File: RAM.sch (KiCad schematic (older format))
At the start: 9 parts

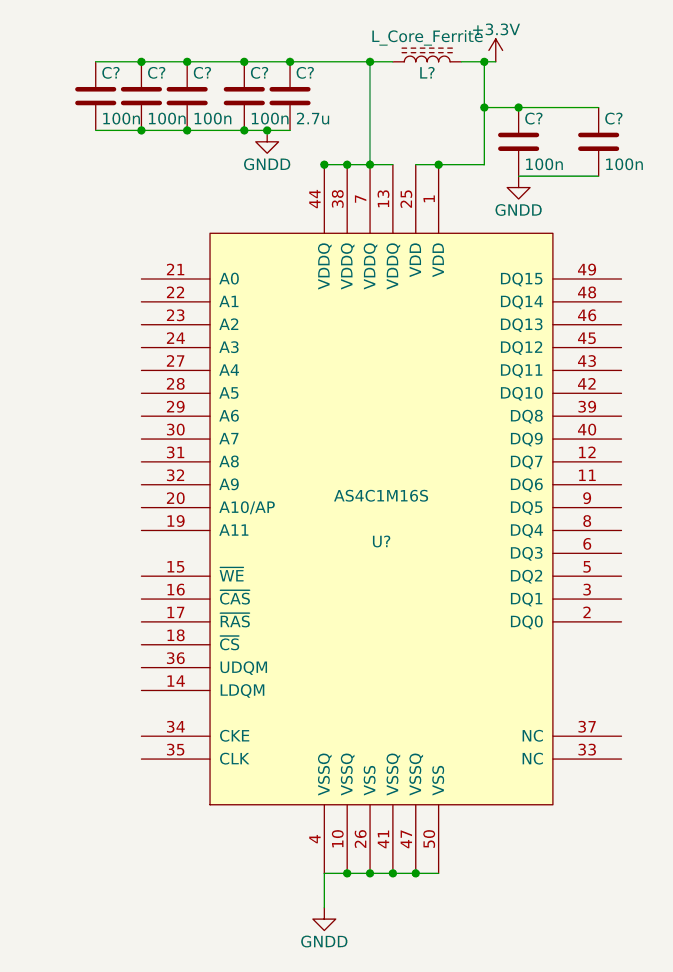
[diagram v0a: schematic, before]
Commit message: Minor fixes and the gitignore was removed
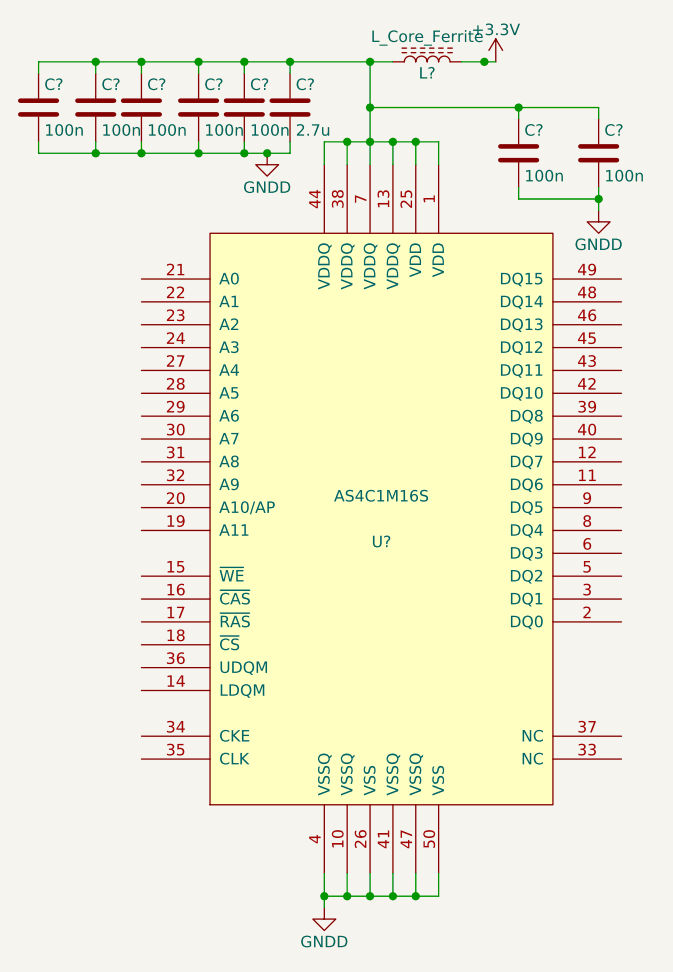
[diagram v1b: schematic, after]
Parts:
- added C?: 100n, symbol C
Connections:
- net +3V3: no longer C?.1, C?.1, U?.1 (VDD), U?.25 (VDD)
- net GNDD: now also C?.2
- net at C?.1, C?.1, C?.1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: now also C?.1, C?.1, U?.1 (VDD), U?.25 (VDD), C?.1
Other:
- moved on the sheet: C?
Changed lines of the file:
@@
 L C C?
 U 1 1 58E1D705
-P 4600 1350
-F 0 "C?" H 4625 1450 50  0000 L CNN
-F 1 "2.7u" H 4625 1250 50  0000 L CNN
-F 2 "" H 4638 1200 50  0001 C CNN
-F 3 "" H 4600 1350 50  0001 C CNN
-	1    4600 1350
+P 4600 1400
+F 0 "C?" H 4625 1500 50  0000 L CNN
+F 1 "2.7u" H 4625 1300 50  0000 L CNN
+F 2 "" H 4638 1250 50  0001 C CNN
+F 3 "" H 4600 1400 50  0001 C CNN
+	1    4600 1400
 	1    0    0    -1
 $EndComp
@@
 L C C?
 U 1 1 58E1D776
-P 4400 1350
-F 0 "C?" H 4425 1450 50  0000 L CNN
-F 1 "100n" H 4425 1250 50  0000 L CNN
-F 2 "" H 4438 1200 50  0001 C CNN
-F 3 "" H 4400 1350 50  0001 C CNN
-	1    4400 1350
+P 4400 1400
+F 0 "C?" H 4425 1500 50  0000 L CNN
+F 1 "100n" H 4425 1300 50  0000 L CNN
+F 2 "" H 4438 1250 50  0001 C CNN
+F 3 "" H 4400 1400 50  0001 C CNN
+	1    4400 1400
 	1    0    0    -1
 $EndComp
@@
 L GNDD #PWR?
 U 1 1 58E1D898
-P 4500 1500
-F 0 "#PWR?" H 4500 1250 50  0001 C CNN
-F 1 "GNDD" H 4500 1350 50  0000 C CNN
-F 2 "" H 4500 1500 50  0001 C CNN
-F 3 "" H 4500 1500 50  0001 C CNN
-	1    4500 1500
+P 4500 1600
+F 0 "#PWR?" H 4500 1350 50  0001 C CNN
+F 1 "GNDD" H 4500 1450 50  0000 C CNN
+F 2 "" H 4500 1600 50  0001 C CNN
+F 3 "" H 4500 1600 50  0001 C CNN
+	1    4500 1600
 	1    0    0    -1
 $EndComp
@@
 	4750 4900 4750 4750
 Wire Wire Line
-	4750 4750 5250 4750
-Connection ~ 4850 4750
-Connection ~ 4950 4750
-Connection ~ 5050 4750
-Connection ~ 5150 4750
-Wire Wire Line
 	5350 1200 5500 1200
 Wire Wire Line
-	3750 1200 5050 1200
+	3500 1200 5050 1200
 Connection ~ 4600 1200
-Wire Wire Line
-	4750 1650 5050 1650
 Wire Wire Line
 	4950 1650 4950 1200
 Connection ~ 4950 1200
-Wire Wire Line
-	5450 1650 5450 1200
 Connection ~ 5450 1200
-Wire Wire Line
-	3750 1500 4600 1500
-Connection ~ 4500 1500
-Connection ~ 4850 1650
+$Comp
+L C C?
+U 1 1 58E1DAA0
+P 3750 1400
+F 0 "C?" H 3775 1500 50  0000 L CNN
+F 1 "100n" H 3775 1300 50  0000 L CNN
+F 2 "" H 3788 1250 50  0001 C CNN
+F 3 "" H 3750 1400 50  0001 C CNN
+	1    3750 1400
+	1    0    0    -1
+$EndComp
+$Comp
+L C C?
+U 1 1 58E1DADF
+P 3950 1400
+F 0 "C?" H 3975 1500 50  0000 L CNN
+F 1 "100n" H 3975 1300 50  0000 L CNN
+F 2 "" H 3988 1250 50  0001 C CNN
+F 3 "" H 3950 1400 50  0001 C CNN
+	1    3950 1400
+	1    0    0    -1
+$EndComp
+$Comp
+L C C?
+U 1 1 58E1DB0D
+P 4200 1400
+F 0 "C?" H 4225 1500 50  0000 L CNN
+F 1 "100n" H 4225 1300 50  0000 L CNN
+F 2 "" H 4238 1250 50  0001 C CNN
+F 3 "" H 4200 1400 50  0001 C CNN
+	1    4200 1400
+	1    0    0    -1
+$EndComp
+Connection ~ 3950 1200
+Connection ~ 4400 1200
+$Comp
+L C C?
+U 1 1 58E1DD36
+P 5600 1600
+F 0 "C?" H 5625 1700 50  0000 L CNN
+F 1 "100n" H 5625 1500 50  0000 L CNN
+F 2 "" H 5638 1450 50  0001 C CNN
+F 3 "" H 5600 1600 50  0001 C CNN
+	1    5600 1600
+	1    0    0    -1
+$EndComp
+$Comp
+L GNDD #PWR?
+U 1 1 58E1DD7E
+P 5950 1850
+F 0 "#PWR?" H 5950 1600 50  0001 C CNN
+F 1 "GNDD" H 5950 1700 50  0000 C CNN
+F 2 "" H 5950 1850 50  0001 C CNN
+F 3 "" H 5950 1850 50  0001 C CNN
+	1    5950 1850
+	1    0    0    -1
+$EndComp
+$Comp
+L C C?
+U 1 1 58E1DDA1
+P 5950 1600
+F 0 "C?" H 5975 1700 50  0000 L CNN
+F 1 "100n" H 5975 1500 50  0000 L CNN
+F 2 "" H 5988 1450 50  0001 C CNN
+F 3 "" H 5950 1600 50  0001 C CNN
+	1    5950 1600
+	1    0    0    -1
+$EndComp
+Wire Wire Line
+	4950 1400 5950 1400
+Connection ~ 5600 1400
+Wire Wire Line
+	3750 1250 3750 1200
+Wire Wire Line
+	3950 1250 3950 1200
+Wire Wire Line
+	4400 1250 4400 1200
+Wire Wire Line
+	4600 1250 4600 1200
+Wire Wire Line
+	4600 1600 4600 1550
+Wire Wire Line
+	3500 1600 4600 1600
+Wire Wire Line
+	3750 1600 3750 1550
+Connection ~ 4500 1600
+Wire Wire Line
+	3950 1550 3950 1600
+Connection ~ 3950 1600
+Wire Wire Line
+	4400 1550 4400 1600
+Connection ~ 4400 1600
+Wire Wire Line
+	4200 1250 4200 1200
+Connection ~ 4200 1200
+Wire Wire Line
+	4200 1550 4200 1600
+Connection ~ 4200 1600
+$Comp
+L C C?
+U 1 1 58DF4B0B
+P 3500 1400
+F 0 "C?" H 3525 1500 50  0000 L CNN
+F 1 "100n" H 3525 1300 50  0000 L CNN
+F 2 "" H 3538 1250 50  0001 C CNN
+F 3 "" H 3500 1400 50  0001 C CNN
+	1    3500 1400
+	1    0    0    -1
+$EndComp
+Wire Wire Line
+	3500 1200 3500 1250
+Connection ~ 3750 1200
+Wire Wire Line
+	3500 1600 3500 1550
+Connection ~ 3750 1600
+Wire Wire Line
+	5600 1450 5600 1400
+Wire Wire Line
+	5950 1400 5950 1450
+Wire Wire Line
+	5950 1750 5950 1850
+Wire Wire Line
+	5950 1800 5600 1800
+Wire Wire Line
+	5600 1800 5600 1750
+Connection ~ 5950 1800
+Wire Wire Line
+	4750 1650 4750 1550
+Wire Wire Line
+	4750 1550 5250 1550
+Connection ~ 4950 1550
+Wire Wire Line
+	5250 1550 5250 1650
+Connection ~ 4950 1400
+Wire Wire Line
+	4850 1650 4850 1550
+Connection ~ 4850 1550
+Wire Wire Line
+	5050 1650 5050 1550
+Connection ~ 5050 1550
+Wire Wire Line
+	5150 1650 5150 1550
+Connection ~ 5150 1550
+Wire Wire Line
+	5250 4750 5250 4850
+Wire Wire Line
+	5250 4850 4750 4850
+Connection ~ 4750 4850
 $Comp
 L AS4C1M16S U?
@@
 	1    0    0    -1
 $EndComp
-Connection ~ 4950 1650
-Wire Wire Line
-	5150 1650 5450 1650
-Connection ~ 5250 1650
-Connection ~ 4750 1650
-$Comp
-L C C?
-U 1 1 58E1DAA0
-P 3750 1350
-F 0 "C?" H 3775 1450 50  0000 L CNN
-F 1 "100n" H 3775 1250 50  0000 L CNN
-F 2 "" H 3788 1200 50  0001 C CNN
-F 3 "" H 3750 1350 50  0001 C CNN
-	1    3750 1350
-	1    0    0    -1
-$EndComp
-$Comp
-L C C?
-U 1 1 58E1DADF
-P 3950 1350
-F 0 "C?" H 3975 1450 50  0000 L CNN
-F 1 "100n" H 3975 1250 50  0000 L CNN
-F 2 "" H 3988 1200 50  0001 C CNN
-F 3 "" H 3950 1350 50  0001 C CNN
-	1    3950 1350
-	1    0    0    -1
-$EndComp
-$Comp
-L C C?
-U 1 1 58E1DB0D
-P 4150 1350
-F 0 "C?" H 4175 1450 50  0000 L CNN
-F 1 "100n" H 4175 1250 50  0000 L CNN
-F 2 "" H 4188 1200 50  0001 C CNN
-F 3 "" H 4150 1350 50  0001 C CNN
-	1    4150 1350
-	1    0    0    -1
-$EndComp
-Connection ~ 3950 1200
-Connection ~ 4150 1200
-Connection ~ 4400 1200
-Connection ~ 3950 1500
-Connection ~ 4400 1500
-Connection ~ 4150 1500
-$Comp
-L C C?
-U 1 1 58E1DD36
-P 5600 1550
-F 0 "C?" H 5625 1650 50  0000 L CNN
-F 1 "100n" H 5625 1450 50  0000 L CNN
-F 2 "" H 5638 1400 50  0001 C CNN
-F 3 "" H 5600 1550 50  0001 C CNN
-	1    5600 1550
-	1    0    0    -1
-$EndComp
-$Comp
-L GNDD #PWR?
-U 1 1 58E1DD7E
-P 5600 1700
-F 0 "#PWR?" H 5600 1450 50  0001 C CNN
-F 1 "GNDD" H 5600 1550 50  0000 C CNN
-F 2 "" H 5600 1700 50  0001 C CNN
-F 3 "" H 5600 1700 50  0001 C CNN
-	1    5600 1700
-	1    0    0    -1
-$EndComp
-$Comp
-L C C?
-U 1 1 58E1DDA1
-P 5950 1550
-F 0 "C?" H 5975 1650 50  0000 L CNN
-F 1 "100n" H 5975 1450 50  0000 L CNN
-F 2 "" H 5988 1400 50  0001 C CNN
-F 3 "" H 5950 1550 50  0001 C CNN
-	1    5950 1550
-	1    0    0    -1
-$EndComp
-Wire Wire Line
-	5600 1700 5950 1700
-Wire Wire Line
-	5450 1400 5950 1400
-Connection ~ 5450 1400
-Connection ~ 5600 1400
+Wire Wire Line
+	4850 4750 4850 4850
+Connection ~ 4850 4850
+Wire Wire Line
+	4950 4750 4950 4850
+Connection ~ 4950 4850
+Wire Wire Line
+	5050 4750 5050 4850
+Connection ~ 5050 4850
+Wire Wire Line
+	5150 4750 5150 4850
+Connection ~ 5150 4850
 $EndSCHEMATC
